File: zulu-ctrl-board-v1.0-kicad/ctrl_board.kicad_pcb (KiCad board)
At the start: 2 copper layers, 79.6 x 45.2 mm, 31 parts, among them J1 Zulu I2C w/ interrupt Connect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, J2 OLED Connector, J3 Conn_01x06_Odd_Even, J5 CENTER_INT, J6 I2C Qwiic, J7 I2C Qwiic, J8 Zulu I2C w/ interrupt Connect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, SW1 SW_SPST, SW2 SW_SPST, SW4 Rotary_Encoder_Switch, U1 PCA9554APW,118

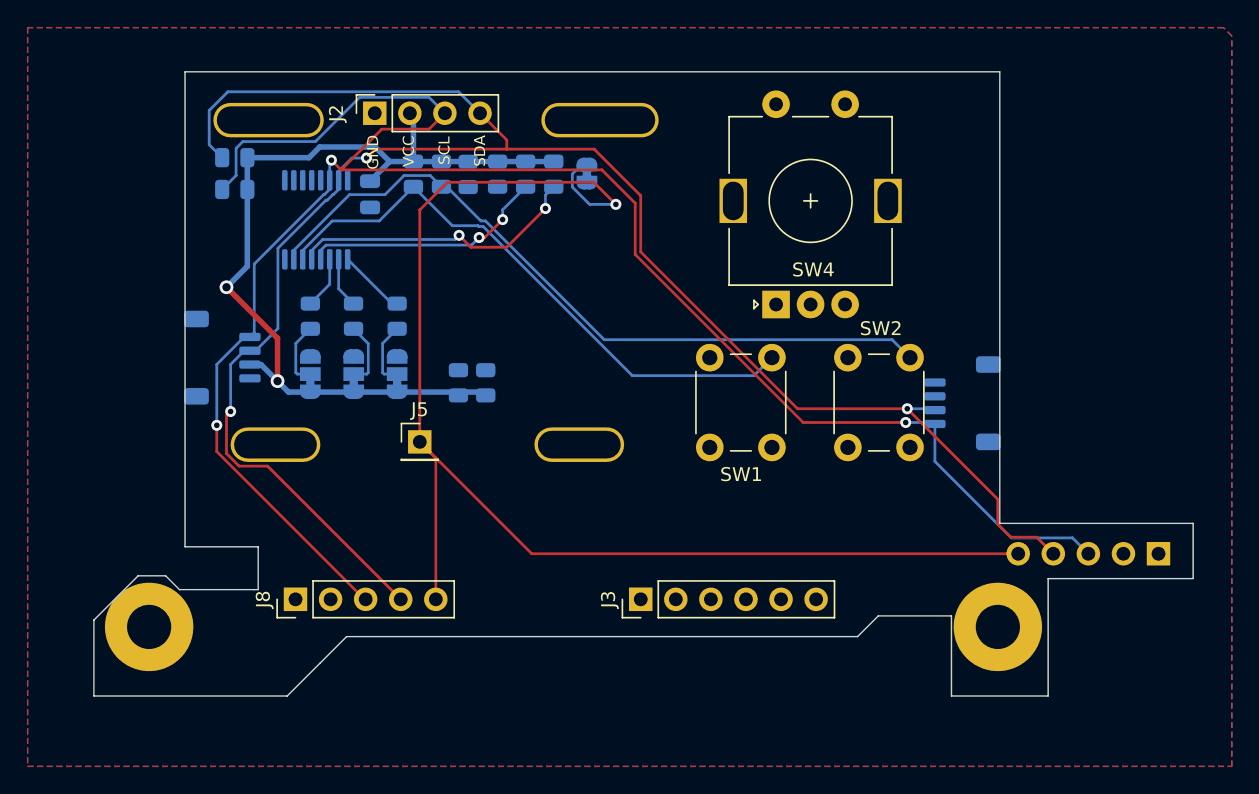
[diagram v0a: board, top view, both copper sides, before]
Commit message: Layout done for the Zulu Control Board v1.0
Layout done for revision 2023a.
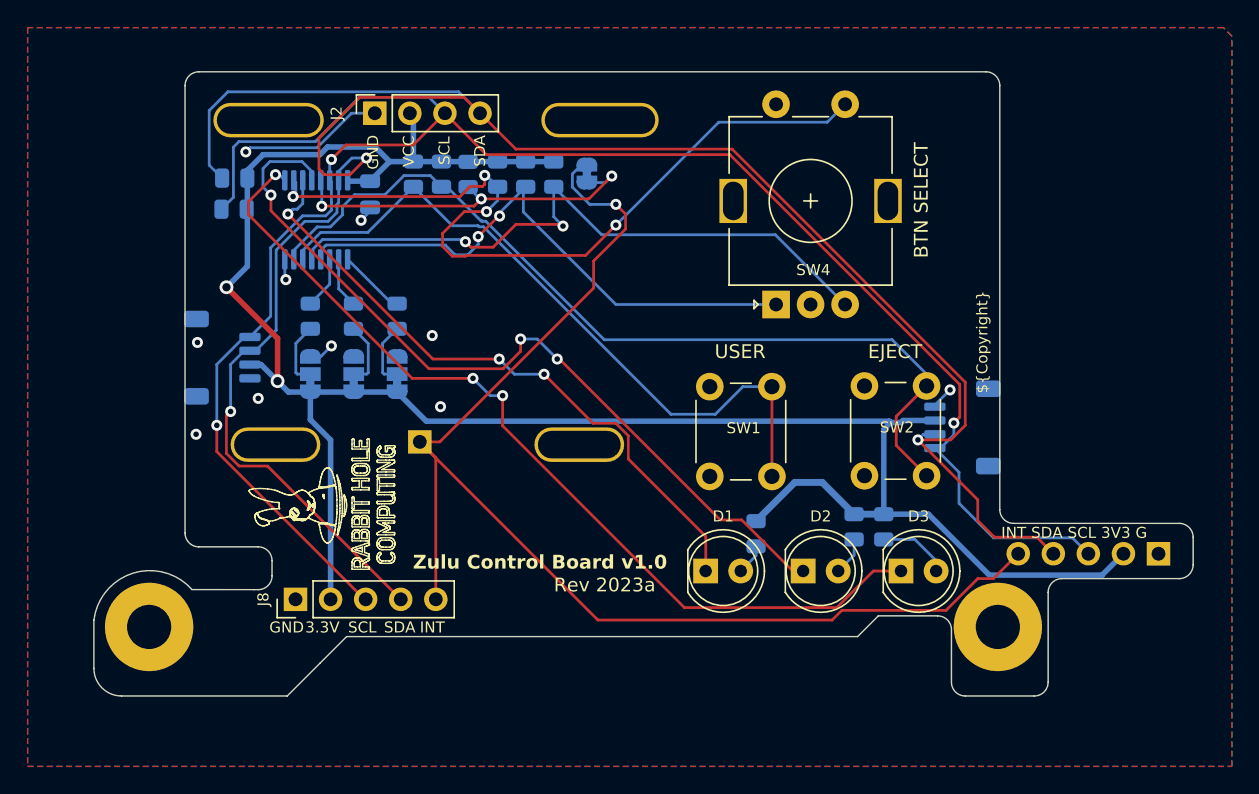
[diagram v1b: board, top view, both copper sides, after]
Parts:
- removed J3: Conn_01x06_Odd_Even, Connector_PinHeader_2.54mm:PinHeader_1x06_P2.54mm_Vertical
- added D1: LED, LED_THT:LED_D5.0mm, F.Cu at (124.7, 190.9)
- added D2: LED, LED_THT:LED_D5.0mm, F.Cu at (131.8, 190.9)
- added D3: LED, LED_THT:LED_D5.0mm, F.Cu at (138.8, 190.9)
- added R14: 10k, Resistor_SMD:R_0805_2012Metric, B.Cu at (137.6, 187.8)
- J5: moved to B.Cu
- J6, J7: footprint Connector_JST:JST_SH_SM04B-SRSS-TB_1x04-1MP_P1.00mm_Horizontal -> mousebites:JST_SH_SM04B-SRSS-TB_1x04-1MP_P1.00mm_Horizontal
- moved R13 28.6 mm to (135.4, 187.8)
- moved R12 24.2 mm to (128.3, 188.2), turned to -90 degrees
- moved SW2 2.38 mm to (136.2, 184.1)
- moved SW1 2.10 mm to (125.0, 184.1)
- moved J6 1.75 mm to (143.3, 180.6)
- moved R11 1.48 mm to (90.6, 162.5)
- moved R10 1.43 mm to (90.5, 164.8)
- turned J5 to 180 degrees
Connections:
- R13 pad 1: +3V3 -> Net-(D2-A)
- R13 pad 2: Net-(J3-Pin_6) -> +3V3
- U1 pad 9: /BUTTON_3 -> /LED_3
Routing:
- net +3V3: track 64.9 -> 153.1 mm
- net /LED_3: track 0.00 -> 66.0 mm, vias 0 -> 3
- net /LED_2: track 0.00 -> 59.6 mm, vias 0 -> 3
- net /BUTTON_4: track 0.00 -> 58.4 mm, vias 0 -> 4
- net /LED_1: track 0.00 -> 46.5 mm, vias 0 -> 3
- net Net-(JP4-A): track 0.00 -> 27.1 mm, vias 0 -> 3
- net /ROTARY_ENC_B: track 21.4 -> 47.9 mm
- net /ROTARY_ENC_A: track 17.8 -> 41.4 mm
- net /SDA: track 139.4 -> 156.2 mm
- net GND: track 0.00 -> 16.7 mm, vias 0 -> 10
- net /BUTTON_2: track 53.0 -> 64.2 mm
- net /BUTTON_1: track 42.7 -> 50.7 mm
- net Net-(D3-A): track 0.00 -> 5.18 mm
- net /INT: track 97.0 -> 93.0 mm
- net Net-(D2-A): track 0.00 -> 2.76 mm
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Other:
- outline, holes or cut-outs redrawn
- board text added: "${Copyright}"
- board text added: "${TITLE}"
- board text added: "2 x M3"
- board text added: "3.3V"
- board text added: "BTN SELECT"
- board text added: "Derived from Tony Kuker's PiSCSI Control Board v1.6 project. Under BSD 3-Clause License Copyright (c) 2020-2023 akuker"
- board text added: "EJECT"
- board text added: "GND"
- board text added: "INT"
- board text added: "INT SDA SCL 3V3 G"
- board text added: "Rev ${REVISION}"
- board text added: "SCL"
- board text added: "SDA"
- board text added: "USER"
